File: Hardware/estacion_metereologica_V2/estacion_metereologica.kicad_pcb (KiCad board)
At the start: 2 copper layers, 21 parts, among them J1 Screw_Terminal_01x02, J2 Step_Down_Mini, J3 Conn_01x03_Pin

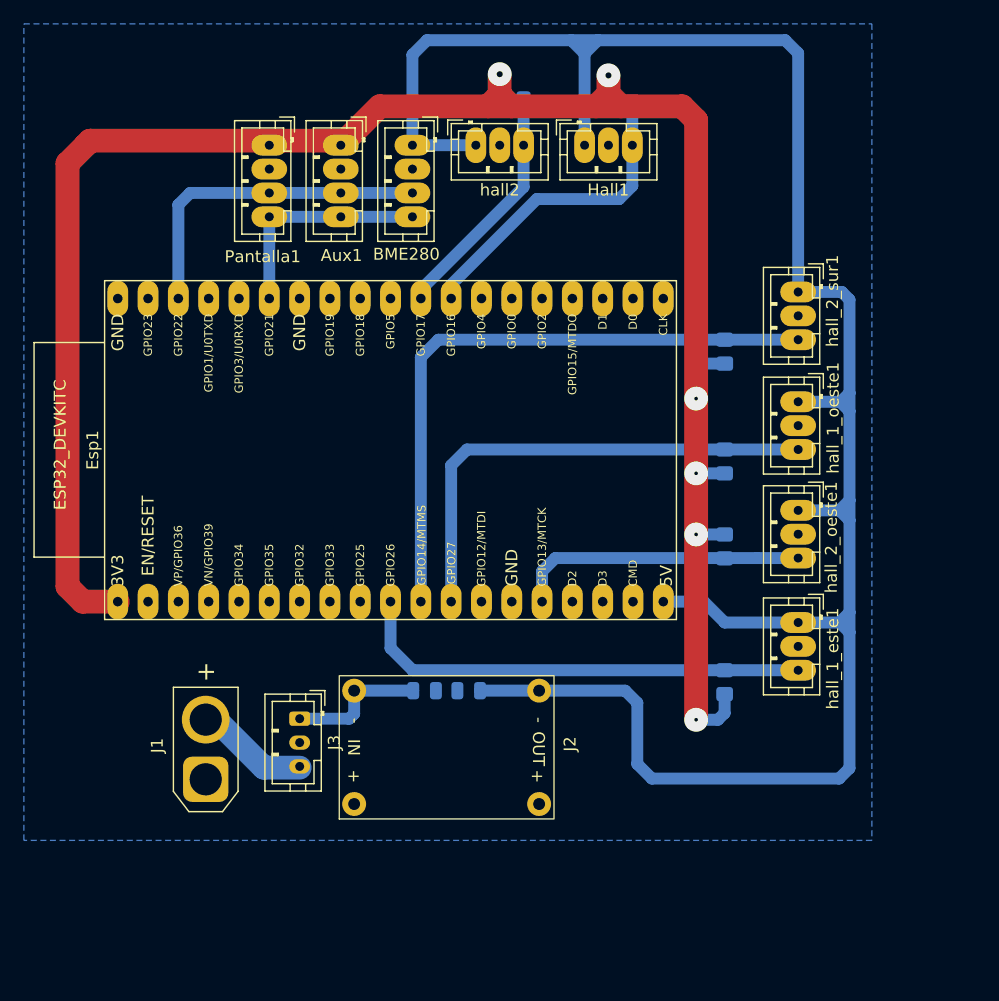
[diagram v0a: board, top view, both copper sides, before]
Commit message: Segunda version del PCB
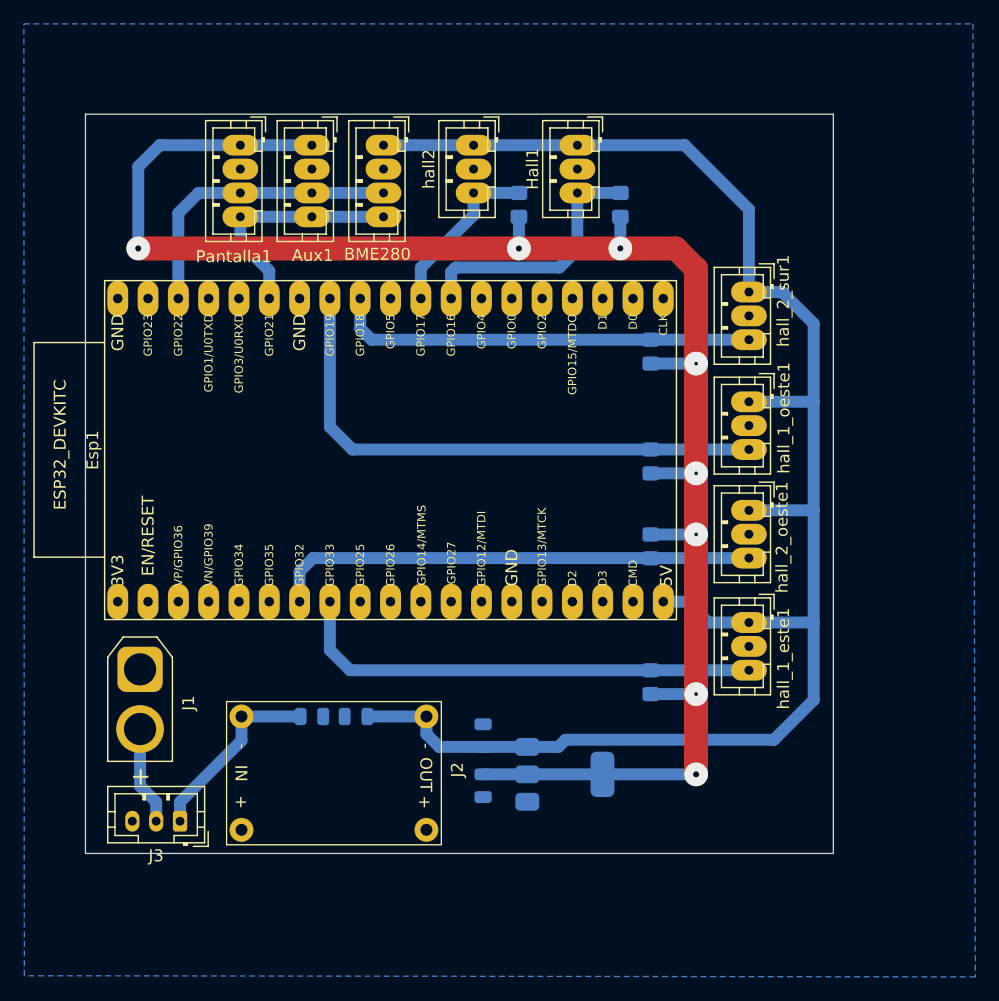
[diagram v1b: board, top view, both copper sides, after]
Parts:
- added C_0.33µF3: C, Capacitor_SMD:C_0805_2012Metric, B.Cu at (58.4, 77.5)
- added C_0.33µF4: C, Capacitor_SMD:C_0805_2012Metric, B.Cu at (58.4, 81.7)
- added U1: AMS1117, Package_TO_SOT_SMD:SOT-223-3_TabPin2, B.Cu at (65.2, 80.7)
- moved J3 13.2 mm to (33.0, 84.7), turned to 180 degrees
- moved J1 10.7 mm to (29.6, 71.9), turned to -90 degrees
- moved C_0.33µF1 9.69 mm to (47.7, 75.9)
- moved C_0.33µF2 9.69 mm to (44.0, 75.9)
- moved J2 9.69 mm to (36.9, 86.6)
- moved R6 8.84 mm to (61.4, 33.0), turned to -90 degrees
- moved R5 8.57 mm to (69.8, 33.0), turned to -90 degrees
- moved R2 6.20 mm to (72.4, 45.3)
- moved R1 6.19 mm to (72.4, 73.0)
- moved R3 6.19 mm to (72.4, 54.5)
- moved R4 6.19 mm to (72.4, 61.6)
- moved hall_1_este1 4.12 mm to (80.6, 68.0)
- moved hall_1_oeste1 4.12 mm to (80.6, 49.5)
- moved hall_2_oeste1 4.12 mm to (80.6, 58.6)
- moved hall_2_sur1 4.12 mm to (80.6, 40.3)
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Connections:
- Esp1 pad 1: 3V3 -> unconnected-(Esp1-3V3-Pad1)
- Esp1 pad 10: OUT_1 -> unconnected-(Esp1-IO26-Pad10)
- Esp1 pad 11: OUT_2 -> unconnected-(Esp1-IO27-Pad11)
- Esp1 pad 12: OUT_3 -> unconnected-(Esp1-IO14-Pad12)
- Esp1 pad 15: OUT_4 -> unconnected-(Esp1-IO13-Pad15)
- Esp1 pad 30: unconnected-(Esp1-IO18-Pad30) -> OUT_2
- Esp1 pad 31: unconnected-(Esp1-IO19-Pad31) -> OUT_3
- Esp1 pad 7: unconnected-(Esp1-IO32-Pad7) -> OUT_4
- Esp1 pad 8: unconnected-(Esp1-IO33-Pad8) -> OUT_1
- J3 pad 2: unconnected-(J3-Pin_2-Pad2) -> Net-(J1-Pin_2)
- J3 pad 3: Net-(J1-Pin_2) -> unconnected-(J3-Pin_3-Pad3)
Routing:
- net 3V3: track 238.8 -> 175.2 mm, vias 6 -> 8
- net VO+: track 187.6 -> 142.9 mm
- net OUT_2: track 52.7 -> 35.5 mm
- net OUT_4: track 24.5 -> 40.6 mm
- net OUT_6: track 20.2 -> 14.4 mm
- net OUT_3: track 41.1 -> 46.7 mm
- net OUT_5: track 26.7 -> 21.6 mm
- net VIN+: track 11.8 -> 16.0 mm
- net SCL: track 27.9 -> 25.1 mm
- net Net-(J1-Pin_2): track 10.0 -> 8.28 mm
- net OUT_1: track 38.8 -> 39.9 mm
- net SDA: track 18.8 -> 19.9 mm
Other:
- board outline added: 62.7 x 61.9 mm
